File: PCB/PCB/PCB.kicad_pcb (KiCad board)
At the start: 2 copper layers, 45.7 x 61 mm, 3 parts, among them M1 Motor_Servo, U1 NodeMCU_1.0_(ESP-12E), U2 DS18B20

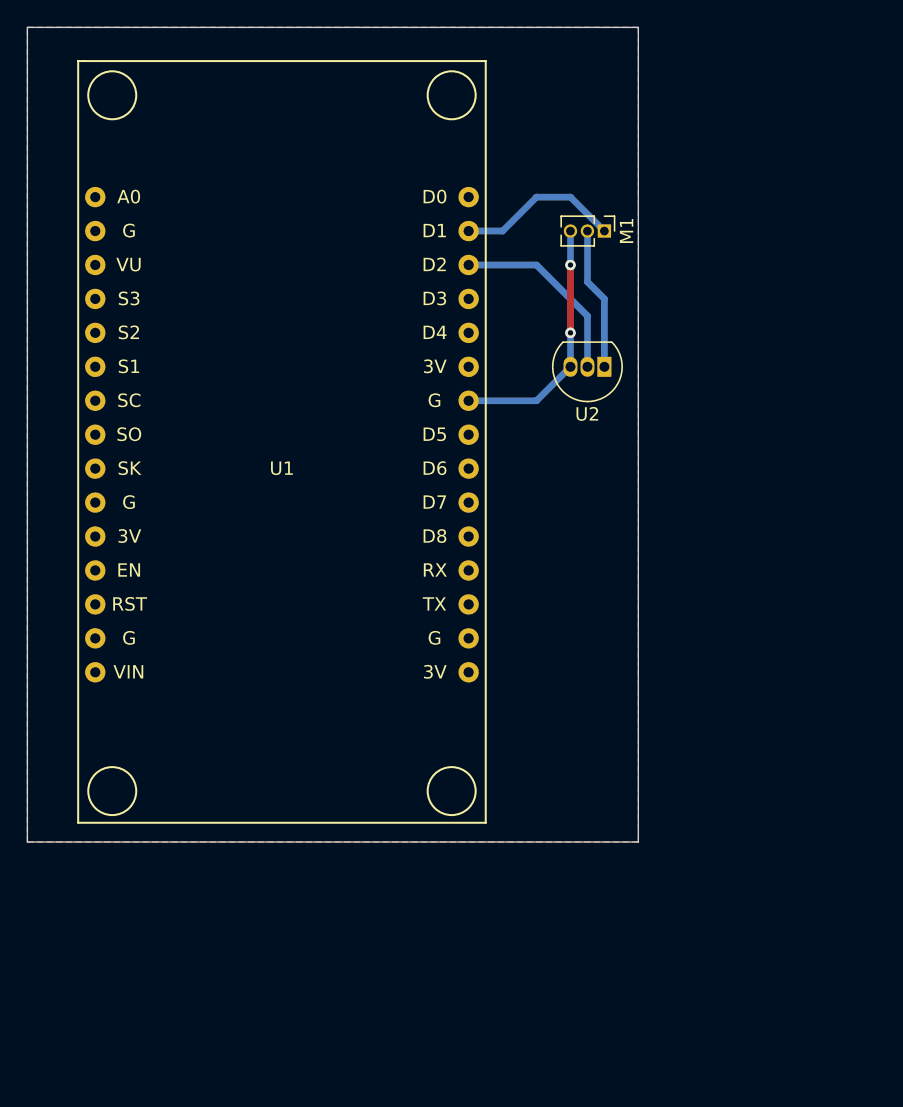
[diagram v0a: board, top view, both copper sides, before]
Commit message: version 1.01
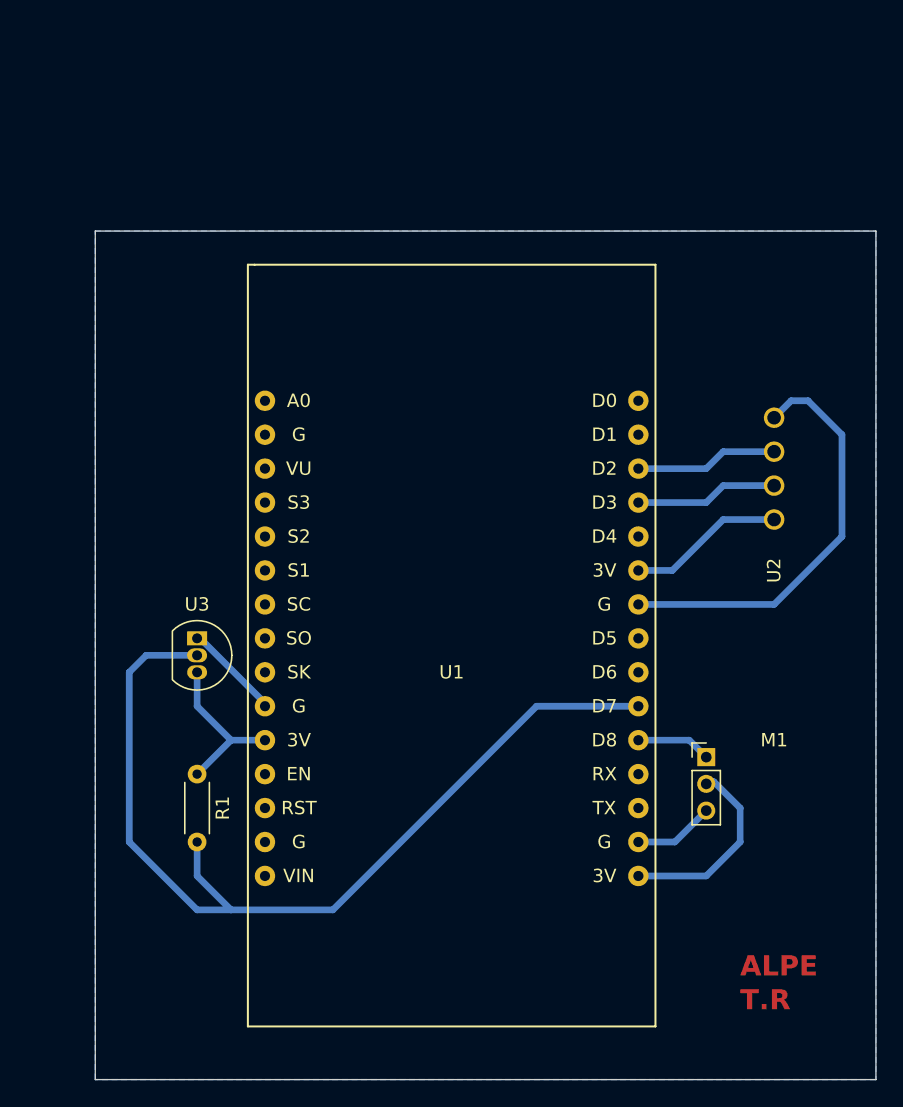
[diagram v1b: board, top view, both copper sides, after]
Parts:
- added R1: 4.7K, Resistor_THT:R_Axial_DIN0204_L3.6mm_D1.6mm_P5.08mm_Horizontal, F.Cu at (129.5, 106.7)
- added U3: DS18B20, Package_TO_SOT_THT:TO-92_Inline, F.Cu at (129.5, 96.5)
- M1: footprint Connector_PinHeader_1.27mm:PinHeader_1x03_P1.27mm_Vertical -> Connector_PinHeader_2.00mm:PinHeader_1x03_P2.00mm_Vertical
- U2: value DS18B20 -> HC-SR04; footprint Package_TO_SOT_THT:TO-92_Inline -> HC-SR04(1):XCVR_HC-SR04
- moved M1 40.1 mm to (167.6, 105.4), turned to 0 degrees
- moved U1 19.8 mm to (148.6, 99.1)
- moved U2 14.8 mm to (172.7, 83.8), turned to 90 degrees
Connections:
- U1 pad 10: unconnected-(U1-GND-Pad10) -> Net-(U3-GND)
- U1 pad 11: unconnected-(U1-3.3V-Pad11) -> Net-(U3-V_{DD})
- U1 pad 16: unconnected-(U1-3.3V-Pad16) -> Net-(M1-+)
- U1 pad 17: unconnected-(U1-GND-Pad17) -> Net-(M1--)
- U1 pad 20: unconnected-(U1-D8(GPIO15)-Pad20) -> Net-(M1-PWM)
- U1 pad 21: unconnected-(U1-D7(GPIO13)-Pad21) -> Net-(U1-D7(GPIO13))
- U1 pad 24: Net-(M1--) -> Net-(U2-GND)
- U1 pad 25: Net-(M1-+) -> Net-(U2-VCC)
- U1 pad 27: unconnected-(U1-D3(GPIO0)-Pad27) -> Net-(U1-D3(GPIO0))
- U1 pad 29: Net-(M1-PWM) -> unconnected-(U1-D1(GPIO5)-Pad29)
- U2 pad 1: Net-(M1-+) -> Net-(U2-VCC)
- U2 pad 2: Net-(U1-D2(GPIO4)) -> Net-(U1-D3(GPIO0))
- U2 pad 3: Net-(M1--) -> Net-(U1-D2(GPIO4))
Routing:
- net Net-(U1-D7(GPIO13)): track 0.00 -> 70.5 mm
- net Net-(U2-GND): track 0.00 -> 31.6 mm
- net Net-(M1--): track 18.8 -> 6.05 mm, vias 2 -> 0
- net Net-(U3-V_{DD}): track 0.00 -> 12.3 mm
- net Net-(U2-VCC): track 0.00 -> 11.7 mm
- net Net-(U1-D3(GPIO0)): track 0.00 -> 10.7 mm
- net Net-(U3-GND): track 0.00 -> 7.32 mm
- net Net-(M1-PWM): track 12.3 -> 5.61 mm
- net Net-(M1-+): track 10.9 -> 14.6 mm
- net Net-(U1-D2(GPIO4)): track 14.3 -> 10.7 mm
- removed copper zone on F.Cu, net (none)
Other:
- board size 45.7 x 61 mm -> 58.4 x 63.5 mm
- board text added: "ALPE"
- board text added: "T.R"
